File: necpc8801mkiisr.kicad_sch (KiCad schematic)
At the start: 216 parts, among them J1 Conn_01x04_MountingPin, SW1 SW_Push, U1 ATmega32U4-MU, Y1 16MHz

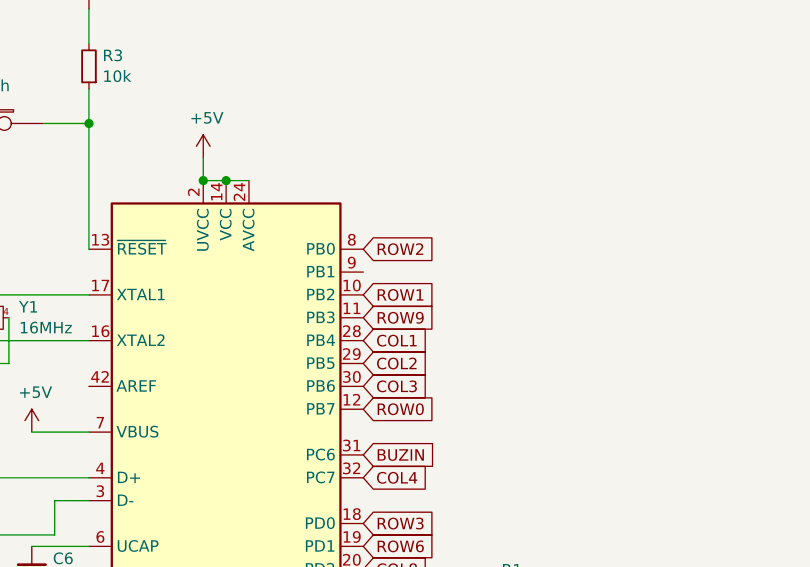
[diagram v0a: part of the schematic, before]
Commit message: updates
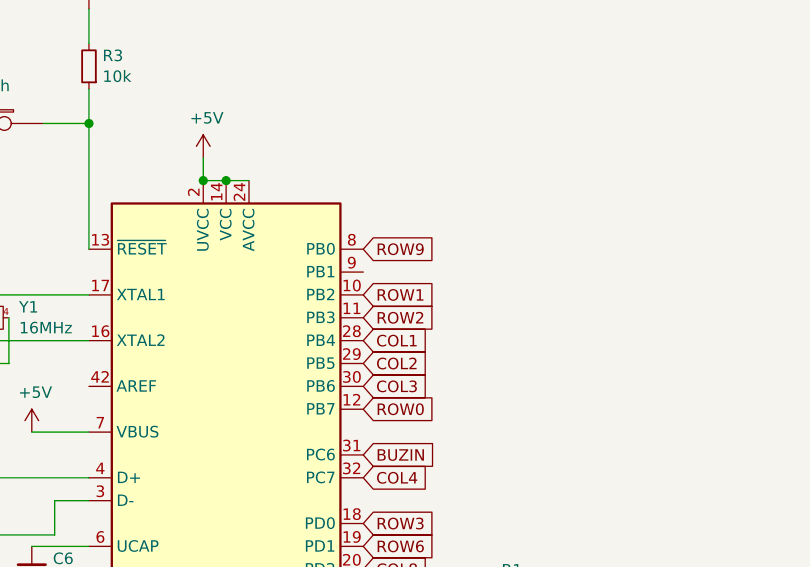
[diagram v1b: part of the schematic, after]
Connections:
- net ROW2: now also U1.11 (PB3); no longer U1.8 (PB0)
- net ROW9: now also U1.8 (PB0); no longer U1.11 (PB3)
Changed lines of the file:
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@@
     (effects (font (size 1.27 1.27)) (justify left bottom))
   )
-  (global_label "ROW2" (shape input) (at 81.28 49.53 0) (fields_autoplaced)
+  (global_label "ROW2" (shape input) (at 81.28 57.15 0) (fields_autoplaced)
     (effects (font (size 1.27 1.27)) (justify left))
-    (property "Intersheetrefs" "${INTERSHEET_REFS}" (at 1.27 -54.61 0)
+    (property "Intersheetrefs" "${INTERSHEET_REFS}" (at 1.27 -46.99 0)
       (effects (font (size 1.27 1.27)) hide)
     )
@@
     )
   )
-  (global_label "ROW9" (shape input) (at 81.28 57.15 0) (fields_autoplaced)
+  (global_label "ROW9" (shape input) (at 81.28 49.53 0) (fields_autoplaced)
     (effects (font (size 1.27 1.27)) (justify left))
-    (property "Intersheetrefs" "${INTERSHEET_REFS}" (at 1.27 -77.47 0)
+    (property "Intersheetrefs" "${INTERSHEET_REFS}" (at 1.27 -85.09 0)
       (effects (font (size 1.27 1.27)) hide)
     )
